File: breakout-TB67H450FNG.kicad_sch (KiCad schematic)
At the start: 12 parts, among them IC1 TB67H450FNG,EL, J1 Conn_01x06, J2 Screw_Terminal_01x02

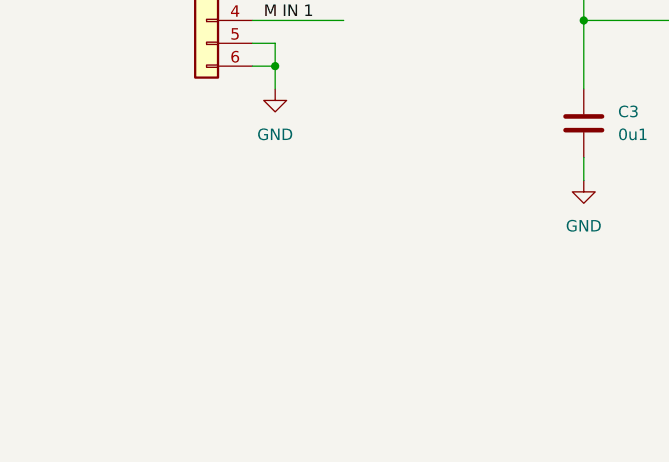
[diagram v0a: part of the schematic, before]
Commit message: Almost close to finishing
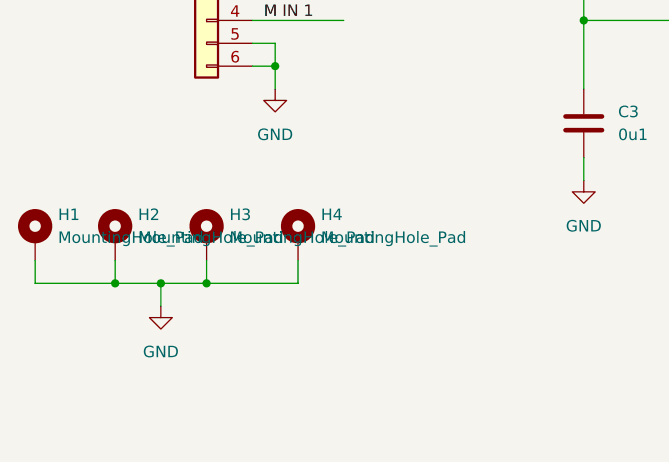
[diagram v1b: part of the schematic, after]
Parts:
- added H1, H2, H3, H4: MountingHole_Pad, MountingHole:MountingHole_3.2mm_M3_Pad_Via, symbol Mechanical:MountingHole_Pad
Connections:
- net GND: now also H1.1, H2.1, H3.1, H4.1
